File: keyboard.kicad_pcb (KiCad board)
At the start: 2 copper layers, 431 x 122.3 mm, 453 parts, among them J2 Conn_01x05_Pin, SW1 SW_Push, U1 STM32F072C8Tx, U2 74AHCT1G125, U3 XC6206PxxxMR, U4 USB6B1

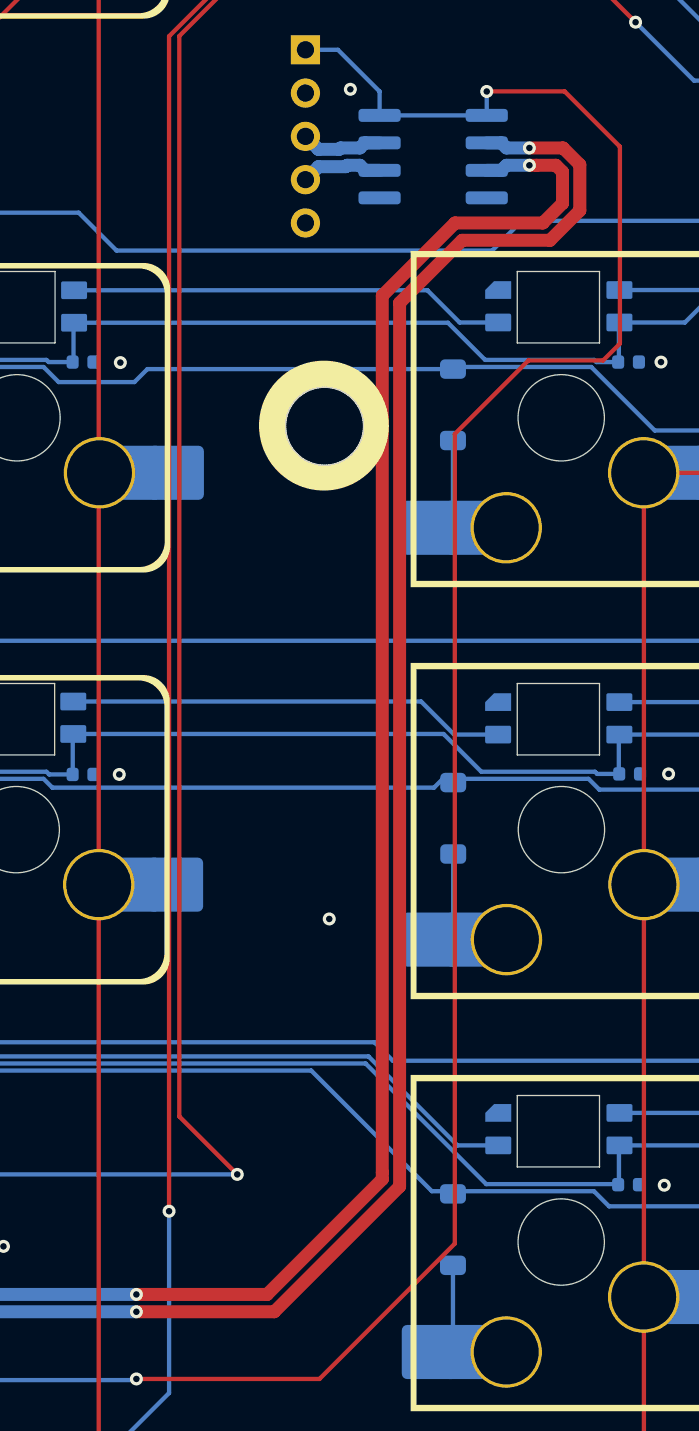
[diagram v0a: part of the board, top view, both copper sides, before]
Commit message: Differential pair length tweak
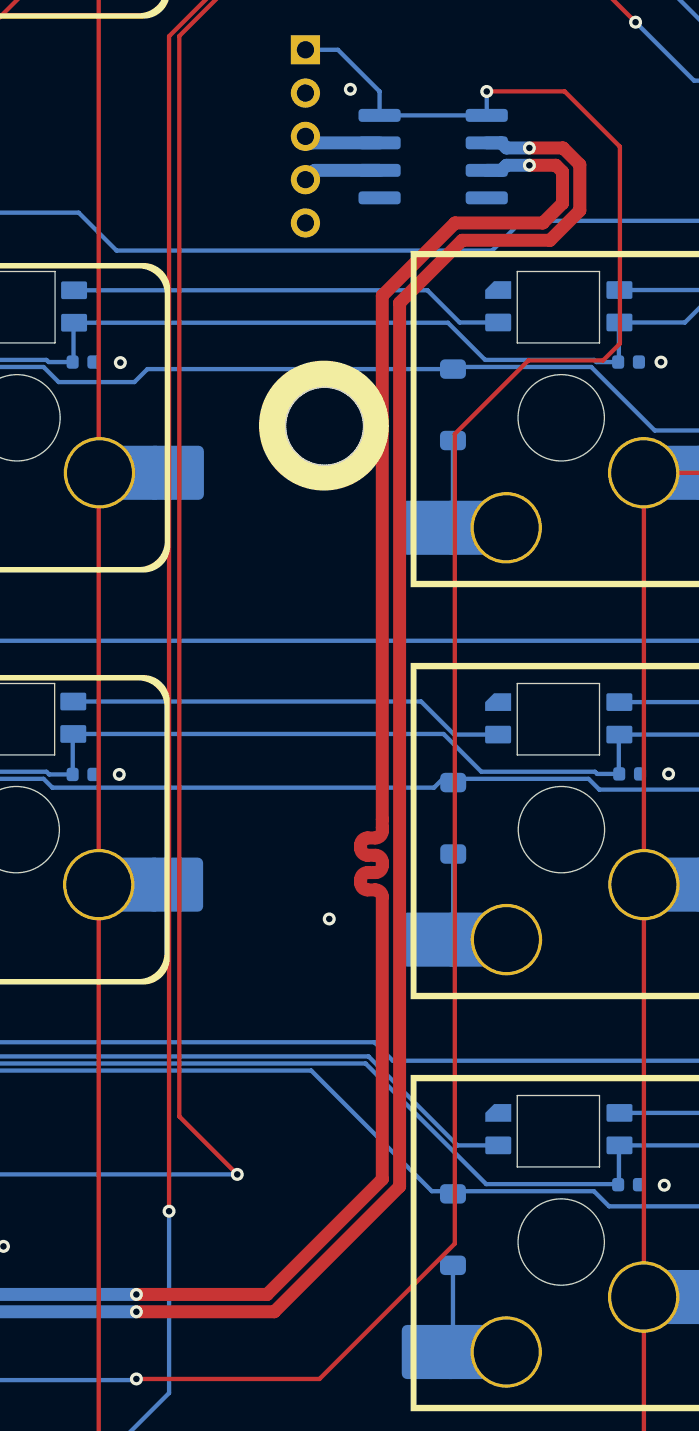
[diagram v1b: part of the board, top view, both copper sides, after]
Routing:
- net D+: track 112.6 -> 115.4 mm
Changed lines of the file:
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@@
 	)
 	(segment
-		(start 375.85 88.959314)
-		(end 375.85 89.275)
+		(start 375.53 74.308392)
+		(end 375.17 74.308392)
 		(width 0.6)
 		(layer "F.Cu")
@@
 	)
 	(segment
-		(start 375.85 89.275)
-		(end 370.529 94.596)
+		(start 375.85 72.649818)
+		(end 375.85 48.459314)
 		(width 0.6)
 		(layer "F.Cu")
@@
 	)
 	(segment
-		(start 379.209314 45.1)
-		(end 375.85 48.459314)
+		(start 375.85 74.788392)
+		(end 375.85 74.628392)
 		(width 0.6)
 		(layer "F.Cu")
@@
 	)
 	(segment
-		(start 384.175 42.740686)
+		(start 383.26863 45.1)
 		(end 384.175 44.19363)
 		(width 0.6)
@@
 	)
 	(segment
+		(start 375.85 89.275)
+		(end 375.85 76.228392)
+		(width 0.6)
+		(layer "F.Cu")
+		(net "D+")
+	)
+	(segment
+		(start 375.85 73.028392)
+		(end 375.85 72.649818)
+		(width 0.6)
+		(layer "F.Cu")
+		(net "D+")
+	)
+	(segment
 		(start 384.175 44.19363)
+		(end 384.175 42.740686)
+		(width 0.6)
+		(layer "F.Cu")
+		(net "D+")
+	)
+	(segment
+		(start 379.209314 45.1)
 		(end 383.26863 45.1)
 		(width 0.6)
@@
 	(segment
 		(start 370.529 94.596)
-		(end 364.49 94.596)
+		(end 375.85 89.275)
 		(width 0.6)
 		(layer "F.Cu")
@@
 	)
 	(segment
-		(start 382.975709 42.435)
-		(end 383.869314 42.435)
+		(start 364.49 94.596)
+		(end 370.529 94.596)
 		(width 0.6)
 		(layer "F.Cu")
@@
 	)
 	(segment
-		(start 375.85 48.459314)
-		(end 375.85 88.959314)
+		(start 375.53 75.908392)
+		(end 375.17 75.908392)
 		(width 0.6)
 		(layer "F.Cu")
@@
 	)
 	(segment
-		(start 382.644338 42.435)
-		(end 382.975709 42.435)
+		(start 375.17 75.108392)
+		(end 375.53 75.108392)
 		(width 0.6)
 		(layer "F.Cu")
@@
 	)
 	(segment
-		(start 383.26863 45.1)
+		(start 375.85 73.188392)
+		(end 375.85 73.028392)
+		(width 0.6)
+		(layer "F.Cu")
+		(net "D+")
+	)
+	(segment
+		(start 374.85 73.988392)
+		(end 374.85 73.828392)
+		(width 0.6)
+		(layer "F.Cu")
+		(net "D+")
+	)
+	(segment
+		(start 374.85 75.588392)
+		(end 374.85 75.428392)
+		(width 0.6)
+		(layer "F.Cu")
+		(net "D+")
+	)
+	(segment
+		(start 375.85 48.459314)
 		(end 379.209314 45.1)
 		(width 0.6)
@@
 	(segment
 		(start 383.869314 42.435)
-		(end 384.175 42.740686)
+		(end 382.644338 42.435)
+		(width 0.6)
+		(layer "F.Cu")
+		(net "D+")
+	)
+	(segment
+		(start 384.175 42.740686)
+		(end 383.869314 42.435)
+		(width 0.6)
+		(layer "F.Cu")
+		(net "D+")
+	)
+	(segment
+		(start 375.17 73.508392)
+		(end 375.53 73.508392)
 		(width 0.6)
 		(layer "F.Cu")
@@
 		(net "D+")
 	)
+	(arc
+		(start 375.17 74.308392)
+		(mid 374.943726 74.214666)
+		(end 374.85 73.988392)
+		(width 0.6)
+		(layer "F.Cu")
+		(net "D+")
+	)
+	(arc
+		(start 375.53 75.108392)
+		(mid 375.756274 75.014666)
+		(end 375.85 74.788392)
+		(width 0.6)
+		(layer "F.Cu")
+		(net "D+")
+	)
+	(arc
+		(start 375.85 74.628392)
+		(mid 375.756274 74.402118)
+		(end 375.53 74.308392)
+		(width 0.6)
+		(layer "F.Cu")
+		(net "D+")
+	)
+	(arc
+		(start 375.17 75.908392)
+		(mid 374.943726 75.814666)
+		(end 374.85 75.588392)
+		(width 0.6)
+		(layer "F.Cu")
+		(net "D+")
+	)
+	(arc
+		(start 374.85 75.428392)
+		(mid 374.943726 75.202118)
+		(end 375.17 75.108392)
+		(width 0.6)
+		(layer "F.Cu")
+		(net "D+")
+	)
+	(arc
+		(start 375.53 73.508392)
+		(mid 375.756274 73.414666)
+		(end 375.85 73.188392)
+		(width 0.6)
+		(layer "F.Cu")
+		(net "D+")
+	)
+	(arc
+		(start 374.85 73.828392)
+		(mid 374.943726 73.602118)
+		(end 375.17 73.508392)
+		(width 0.6)
+		(layer "F.Cu")
+		(net "D+")
+	)
+	(arc
+		(start 375.85 76.228392)
+		(mid 375.756274 76.002118)
+		(end 375.53 75.908392)
+		(width 0.6)
+		(layer "F.Cu")
+		(net "D+")
+	)
 	(segment
 		(start 364.49 94.596)
@@
 	)
 	(segment
-		(start 374.225 42.435)
-		(end 374.815 42.435)
-		(width 0.6)
-		(layer "B.Cu")
-		(net "DIn+")
-	)
-	(segment
-		(start 374.815 42.435)
-		(end 375.05 42.67)
+		(start 372.73 42.67)
+		(end 372.3 43.1)
 		(width 0.6)
 		(layer "B.Cu")
@@
 	)
 	(segment
-		(start 374.16 42.5)
-		(end 374.225 42.435)
+		(start 375.725 42.67)
+		(end 372.73 42.67)
 		(width 0.6)
 		(layer "B.Cu")
@@
 	)
 	(segment
-		(start 372.9 42.5)
-		(end 374.16 42.5)
-		(width 0.6)
-		(layer "B.Cu")
-		(net "DIn+")
-	)
-	(segment
-		(start 375.05 42.67)
-		(end 375.725 42.67)
-		(width 0.6)
-		(layer "B.Cu")
-		(net "DIn+")
-	)
-	(segment
-		(start 372.3 43.1)
-		(end 372.9 42.5)
-		(width 0.6)
-		(layer "B.Cu")
-		(net "DIn+")
-	)
-	(segment
-		(start 374.815 41.635)
-		(end 375.05 41.4)
-		(width 0.6)
-		(layer "B.Cu")
-		(net "DIn-")
-	)
-	(segment
-		(start 373.853856 41.7)
-		(end 373.918856 41.635)
+		(start 375.725 41.4)
+		(end 372.6 41.4)
 		(width 0.6)
 		(layer "B.Cu")
@@
 	)
 	(segment
-		(start 373.918856 41.635)
-		(end 374.815 41.635)
-		(width 0.6)
-		(layer "B.Cu")
-		(net "DIn-")
-	)
-	(segment
-		(start 372.3 41.1)
-		(end 372.9 41.7)
-		(width 0.6)
-		(layer "B.Cu")
-		(net "DIn-")
-	)
-	(segment
-		(start 375.05 41.4)
-		(end 375.725 41.4)
-		(width 0.6)
-		(layer "B.Cu")
-		(net "DIn-")
-	)
-	(segment
-		(start 372.9 41.7)
-		(end 373.853856 41.7)
+		(start 372.6 41.4)
+		(end 372.3 41.1)
 		(width 0.6)
 		(layer "B.Cu")
@@
 		(members "faf74561-e777-49ac-b434-80f66b7b5f86")
 	)
+	(generated
+		(type tuning_pattern)
+		(name "Tuning Pattern")
+		(layer "F.Cu")
+		(base_line
+			(pts
+				(xy 375.85 76.228392) (xy 375.85 72.649818)
+			)
+		)
+		(corner_radius_percent 80)
+		(end
+			(xy 375.85 72.649818)
+		)
+		(initial_side "left")
+		(is_time_domain no)
+		(last_diff_pair_gap 0.18)
+		(last_netname "D+")
+		(last_status "tuned")
+		(last_track_width 0.6)
+		(last_tuning_length 118.575442)
+		(max_amplitude 1)
+		(min_amplitude 0.2)
+		(min_spacing 0.6)
+		(origin
+			(xy 375.85 76.228392)
+		)
+		(override_custom_rules no)
+		(rounded yes)
+		(single_sided no)
+		(target_delay 1000000)
+		(target_delay_max 1000000)
+		(target_delay_min 0)
+		(target_length 1000000)
+		(target_length_max 1000000)
+		(target_length_min 0)
+		(target_skew 0)
+		(target_skew_max 0.1)
+		(target_skew_min -0.1)
+		(tuning_mode "single")
+		(members "152cdca4-bfcc-498f-975f-8be19472034a" "17858806-3853-4025-a193-c9de21fccbba"
+			"1ce5a72b-8873-4abe-835b-c5e57b44963b" "1d17cf02-8da2-4a27-b68f-f4fcaa81fbef"
+			"228a2b4a-a2ec-4e86-89c4-02da1f133986" "40c289c0-f887-49ba-a167-5a40f5e5bfb5"
+			"597b9ad1-c064-4b83-ac44-c2554ee8fcf5" "5d15edfc-8f2b-4363-8ade-d0ebbc74ce22"
+			"624e195d-b42b-4180-873b-e0b2a79b14cd" "a7717af8-7039-4e70-b00e-1538053dcd6b"
+			"b994ea88-2696-45b4-94f0-ee8e0b38dfa2" "be29fb73-72d9-4f4a-9de1-113db438335b"
+			"d4ff5187-a9e5-4038-829d-068d625337bb" "d86fcc4e-8420-4592-9644-51d7dc238d46"
+			"e30b1e98-4435-4200-b8a2-e4356eeb4b5c" "f1629ca2-da9b-4db6-9076-83c9e1598a44"
+			"fea5637a-e850-47a9-9f87-e35b3149cb7d"
+		)
+	)
 	(embedded_fonts no)
